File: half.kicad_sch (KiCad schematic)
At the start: 88 parts, among them J3 JST_PH, Q1 Q_PMOS_GSD, SW1 SW_Push, SW13 SW_Push, SW14 SW_Push, SW15 SW_Push, SW16 SW_Push, SW17 SW_Push, SW18 SW_Push, SW25 SW_Push, SW26 SW_Push, SW27 SW_Push, SW28 SW_Push, SW29 SW_Push, SW3 SW_Push, SW30 SW_Push, SW37 SW_Push, SW38 SW_Push, SW39 SW_Push, SW40 SW_Push, SW41 SW_Push, SW42 SW_Push, SW49 SW_Push, SW5 SW_Push, SW50 SW_Push, SW51 SW_Push, SW52 SW_Push, SW53 SW_Push, SW54 RotaryEncoder_Switch, SW61 SW_SPDT, SW7 SW_Push, SW8 SW_Push, SW9 SW_Push, U3 SuperMini nRF52840

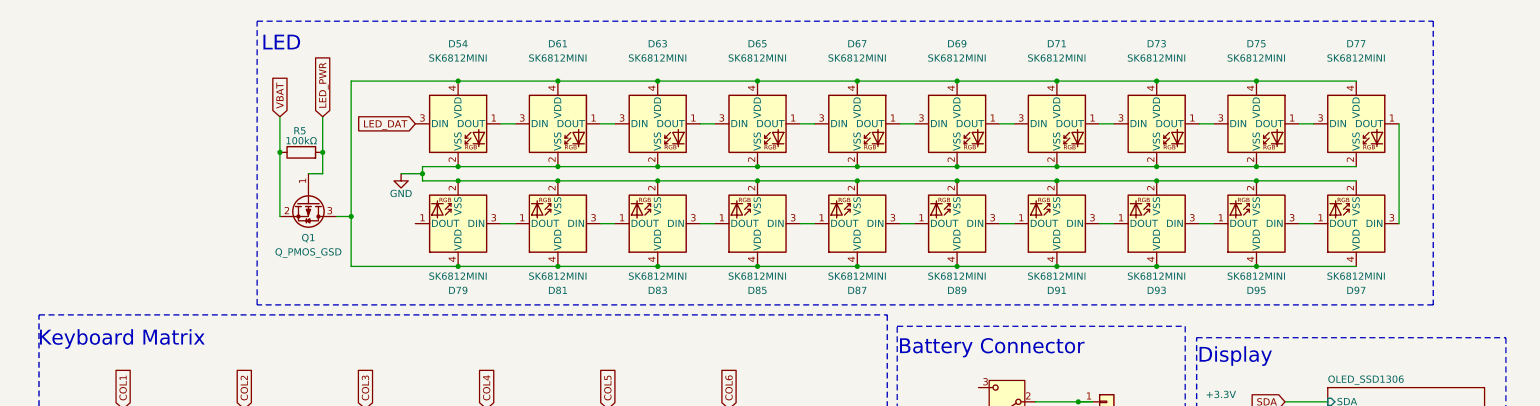
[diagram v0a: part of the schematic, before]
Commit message: update
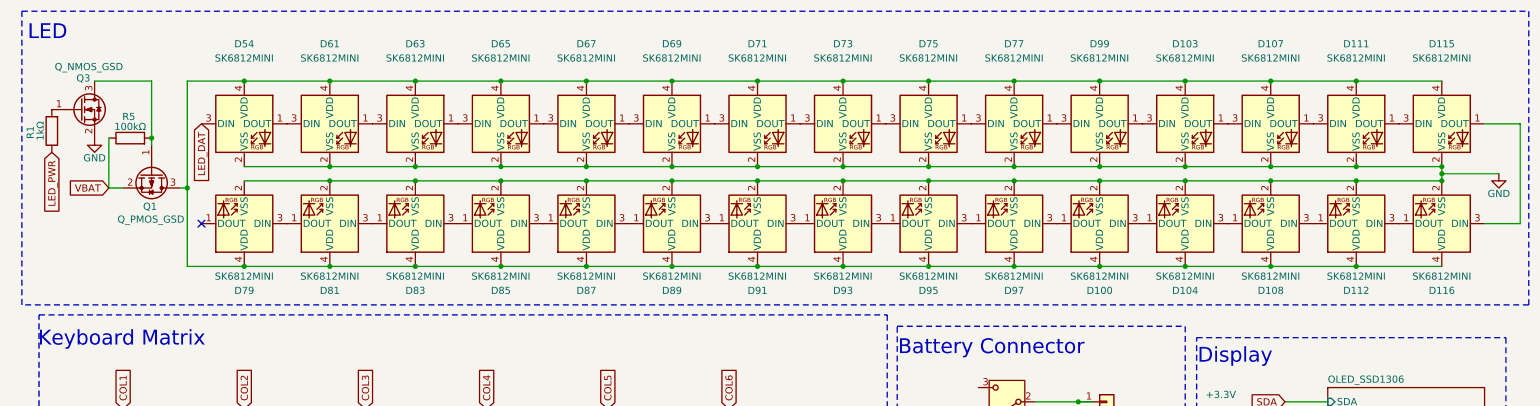
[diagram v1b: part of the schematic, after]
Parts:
- added D100, D103, D104, D107, D108, D111, D112, D115, D116, D99: SK6812MINI, LED_SMD:LED_SK6812MINI_PLCC4_3.5x3.5mm_P1.75mm, symbol LED:SK6812MINI
- added Q3: Q_NMOS_GSD, symbol Transistor_FET:Q_NMOS_GSD
- added R1: 1kΩ, Resistor_SMD:R_0805_2012Metric, symbol Device:R
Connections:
- net GND: now also D100.2 (VSS), D103.2 (VSS), D104.2 (VSS), D107.2 (VSS), D108.2 (VSS), D111.2 (VSS), D112.2 (VSS), D115.2 (VSS), D116.2 (VSS), D99.2 (VSS), Q3.2 (S)
- net LED_PWR: now also R1.1; no longer Q1.1 (G), R5.2
- net at D54.4 (VDD), D61.4 (VDD), D63.4 (VDD)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: now also D100.4 (VDD), D103.4 (VDD), D104.4 (VDD), D107.4 (VDD), D108.4 (VDD), D111.4 (VDD), D112.4 (VDD), D115.4 (VDD), D116.4 (VDD), D99.4 (VDD)
- net at D77.1 (DOUT): now also D99.3 (DIN); no longer D97.3 (DIN)
- new net: D100.3 (DIN), D104.1 (DOUT)
- new net: D104.3 (DIN), D108.1 (DOUT)
- new net: Q3.1 (G), R1.2
- new net: Q1.1 (G), Q3.3 (D), R5.2
- new net: D103.3 (DIN), D99.1 (DOUT)
- new net: D112.3 (DIN), D116.1 (DOUT)
- new net: D115.1 (DOUT), D116.3 (DIN)
- new net: D107.1 (DOUT), D111.3 (DIN)
- new net: D103.1 (DOUT), D107.3 (DIN)
- new net: D111.1 (DOUT), D115.3 (DIN)
- new net: D108.3 (DIN), D112.1 (DOUT)
- new net: D100.1 (DOUT), D97.3 (DIN)
- no-connect marks 0 -> 1
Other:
- moved on the sheet: D54, D61, D63, D65, D67, D69, D71, D73, D75, D77, D79, D81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
